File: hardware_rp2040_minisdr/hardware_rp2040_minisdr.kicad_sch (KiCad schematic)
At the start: 48 parts, among them IC1 PSA4-5043+, IC2 ADE-11X+, IC3 SI5351A-B-GTR, IC4 GALI-84+, IC5 ADCS7476AIMFX_NOPB, J1 Conn_Coaxial_Small, J2 USB_A, SW1 SW_Push, U1 RP2040, U2 W25Q128JVS, U3 AMS1117-3.3, Y1 Crystal_GND24, Y2 Crystal_GND24

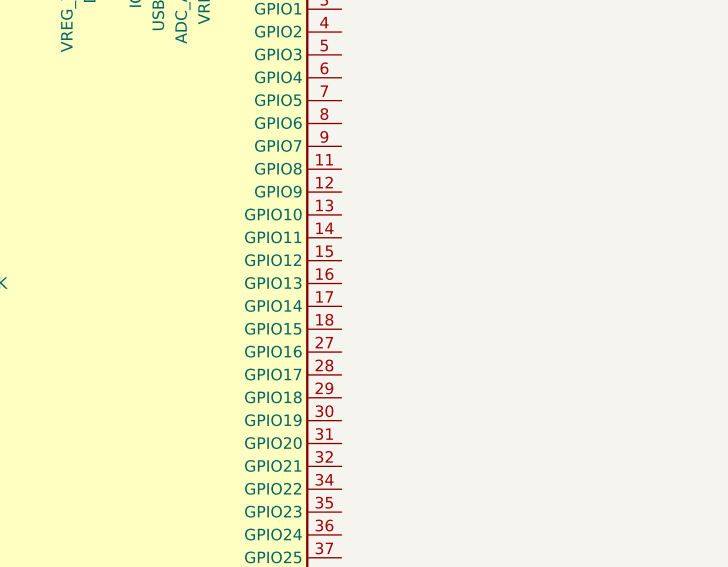
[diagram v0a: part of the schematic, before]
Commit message: board
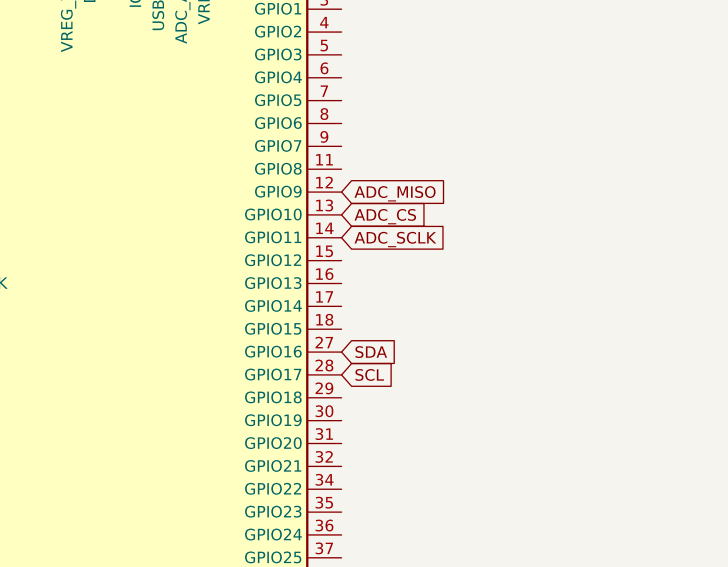
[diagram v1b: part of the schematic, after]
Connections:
- net ADC_CS: now also U1.13 (GPIO10)
- net ADC_MISO: now also U1.12 (GPIO9)
- net ADC_SCLK: now also U1.14 (GPIO11)
- net SCL: now also U1.28 (GPIO17)
- net SDA: now also U1.27 (GPIO16)
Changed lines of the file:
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@@
+		)
+	)
+	(global_label "ADC_SCLK"
+		(shape input)
+		(at 228.6 96.52 0)
+		(fields_autoplaced yes)
+		(effects
+			(font
+				(size 1.27 1.27)
+			)
+			(justify left)
+		)
+		(property "Intersheetrefs" "${INTERSHEET_REFS}"
+			(at 240.959 96.52 0)
+			(effects
+				(font
+					(size 1.27 1.27)
+				)
+				(justify left)
+				(hide yes)
+			)
 		)
 	)
@@
 		)
 	)
+	(global_label "ADC_CS"
+		(shape input)
+		(at 228.6 93.98 0)
+		(fields_autoplaced yes)
+		(effects
+			(font
+				(size 1.27 1.27)
+			)
+			(justify left)
+		)
+		(property "Intersheetrefs" "${INTERSHEET_REFS}"
+			(at 238.6609 93.98 0)
+			(effects
+				(font
+					(size 1.27 1.27)
+				)
+				(justify left)
+				(hide yes)
+			)
+		)
+	)
+	(global_label "SCL"
+		(shape input)
+		(at 228.6 111.76 0)
+		(fields_autoplaced yes)
+		(effects
+			(font
+				(size 1.27 1.27)
+			)
+			(justify left)
+		)
+		(property "Intersheetrefs" "${INTERSHEET_REFS}"
+			(at 235.0928 111.76 0)
+			(effects
+				(font
+					(size 1.27 1.27)
+				)
+				(justify left)
+				(hide yes)
+			)
+		)
+	)
+	(global_label "ADC_MISO"
+		(shape input)
+		(at 228.6 91.44 0)
+		(fields_autoplaced yes)
+		(effects
+			(font
+				(size 1.27 1.27)
+			)
+			(justify left)
+		)
+		(property "Intersheetrefs" "${INTERSHEET_REFS}"
+			(at 240.7776 91.44 0)
+			(effects
+				(font
+					(size 1.27 1.27)
+				)
+				(justify left)
+				(hide yes)
+			)
+		)
+	)
 	(global_label "GND"
 		(shape input)
@@
 				(hide yes)
 			)
+		)
+	)
+	(global_label "SDA"
+		(shape input)
+		(at 228.6 109.22 0)
+		(fields_autoplaced yes)
+		(effects
+			(font
+				(size 1.27 1.27)
+			)
+			(justify left)
+		)
+		(property "Intersheetrefs" "${INTERSHEET_REFS}"
+			(at 235.1533 109.22 0)
+			(effects
+				(font
+					(size 1.27 1.27)
+				)
+				(justify left)
+				(hide yes)
+			)

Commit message: board
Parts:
- C10, C11, C12, C13, C14, C15, C17, C18, C2, C20, C21, C23, C24, C25, C26, C3, C6, C7, C9: footprint (none) -> Capacitor_SMD:C_0402_1005Metric
- D1: footprint SOT95P280X145-5N -> (none)
- IC1: footprint PSA45043 -> (none)
- IC2: footprint SOTFL254P691X284-6N -> (none)
- IC3: footprint SOP50P490X110-10N -> (none)
- IC4: footprint GALI5 -> (none)
- IC5: footprint SOT95P280X145-6N -> (none)
- J1: footprint (none) -> Connector_Coaxial:SMA_Amphenol_132289_EdgeMount
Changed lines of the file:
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@@
 			)
 		)
-		(property "Footprint" "SOP50P490X110-10N"
+		(property "Footprint" ""
 			(at 153.67 243.51 0)
 			(effects
@@
 			)
 		)
-		(property "Footprint" ""
+		(property "Footprint" "Connector_Coaxial:SMA_Amphenol_132289_EdgeMount"
 			(at 29.21 106.68 0)
 			(effects
@@
 			)
 		)
-		(property "Footprint" ""
+		(property "Footprint" "Capacitor_SMD:C_0402_1005Metric"
 			(at 247.3452 44.45 0)
 			(effects
@@
 			)
 		)
-		(property "Footprint" ""
+		(property "Footprint" "Capacitor_SMD:C_0402_1005Metric"
 			(at 77.1652 130.81 0)
 			(effects
@@
 			)
 		)
-		(property "Footprint" ""
+		(property "Footprint" "Capacitor_SMD:C_0402_1005Metric"
 			(at 224.4852 44.45 0)
 			(effects
@@
 			)
 		)
-		(property "Footprint" "PSA45043"
+		(property "Footprint" ""
 			(at 45.72 14.3 0)
 			(effects
@@
 			)
 		)
-		(property "Footprint" "SOT95P280X145-5N"
+		(property "Footprint" ""
 			(at 55.88 172.39 0)
 			(effects
@@
 			)
 		)
-		(property "Footprint" ""
+		(property "Footprint" "Capacitor_SMD:C_0402_1005Metric"
 			(at 155.9052 133.35 0)
 			(effects
@@
 			)
 		)
-		(property "Footprint" "SOTFL254P691X284-6N"
+		(property "Footprint" ""
 			(at 72.39 213.03 0)
 			(effects
@@
 			)
 		)
-		(property "Footprint" ""
+		(property "Footprint" "Capacitor_SMD:C_0402_1005Metric"
 			(at 39.37 133.6548 0)
 			(effects
@@
 			)
 		)
-		(property "Footprint" ""
+		(property "Footprint" "Capacitor_SMD:C_0402_1005Metric"
 			(at 254.9652 44.45 0)
 			(effects
@@
 			)
 		)
-		(property "Footprint" "SOT95P280X145-6N"
+		(property "Footprint" ""
 			(at 66.04 251.13 0)
 			(effects
@@
 			)
 		)
-		(property "Footprint" ""
+		(property "Footprint" "Capacitor_SMD:C_0402_1005Metric"
 			(at 239.7252 44.45 0)
 			(effects
@@
 			)
 		)
-		(property "Footprint" "GALI5"
+		(property "Footprint" ""
 			(at 91.44 32.08 0)
 			(effects
@@
 			)
 		)
-		(property "Footprint" ""
+		(property "Footprint" "Capacitor_SMD:C_0402_1005Metric"
 			(at 262.5852 44.45 0)
 			(effects
@@
 			)
 		)
-		(property "Footprint" ""
+		(property "Footprint" "Capacitor_SMD:C_0402_1005Metric"
 			(at 187.6552 48.26 0)
 			(effects
@@
 			)
 		)
-		(property "Footprint" ""
+		(property "Footprint" "Capacitor_SMD:C_0402_1005Metric"
 			(at 29.5148 147.32 0)
 			(effects
@@
 			)
 		)
-		(property "Footprint" ""
+		(property "Footprint" "Capacitor_SMD:C_0402_1005Metric"
 			(at 108.9152 162.56 0)
 			(effects
@@
 			)
 		)
-		(property "Footprint" ""
+		(property "Footprint" "Capacitor_SMD:C_0402_1005Metric"
 			(at 195.2752 48.26 0)
 			(effects
@@
 			)
 		)
-		(property "Footprint" ""
+		(property "Footprint" "Capacitor_SMD:C_0402_1005Metric"
 			(at 216.8652 44.45 0)
 			(effects
@@
 			)
 		)
-		(property "Footprint" ""
+		(property "Footprint" "Capacitor_SMD:C_0402_1005Metric"
 			(at 38.1 105.7148 0)
 			(effects
@@
 			)
 		)
-		(property "Footprint" ""
+		(property "Footprint" "Capacitor_SMD:C_0402_1005Metric"
 			(at 106.68 108.2548 0)
 			(effects
@@
 			)
 		)
-		(property "Footprint" ""
+		(property "Footprint" "Capacitor_SMD:C_0402_1005Metric"
 			(at 132.3848 127 0)
 			(effects
@@
 			)
 		)
-		(property "Footprint" ""
+		(property "Footprint" "Capacitor_SMD:C_0402_1005Metric"
 			(at 108.9152 147.32 0)
 			(effects
@@
 			)
 		)
-		(property "Footprint" ""
+		(property "Footprint" "Capacitor_SMD:C_0402_1005Metric"
 			(at 232.1052 44.45 0)
 			(effects
@@
 			)
 		)
-		(property "Footprint" ""
+		(property "Footprint" "Capacitor_SMD:C_0402_1005Metric"
 			(at 155.9052 114.3 0)
 			(effects

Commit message: board
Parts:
- C16, C8: footprint (none) -> Capacitor_SMD:C_0402_1005Metric
- C19, C22, C4, C5: footprint (none) -> Capacitor_SMD:C_0805_2012Metric
- D1: footprint (none) -> user_imported_devices:ESDS314BVR_SOT95P280X145-5N
- IC1: footprint (none) -> user_imported_devices:PSA45043
- IC2: footprint (none) -> user_imported_devices:ADE-11X+_SOTFL254P691X284-6N
- IC3: footprint (none) -> user_imported_devices:SI5351_SOP50P490X110-10N
- IC4: footprint (none) -> user_imported_devices:GALI5
- IC5: footprint (none) -> user_imported_devices:ADCS7476_SOT95P280X145-6N
- L1, L2, L3, L4: footprint (none) -> Inductor_SMD:L_0805_2012Metric
- R2, R3, R4, R5, R6: footprint (none) -> Resistor_SMD:R_0402_1005Metric
- SW1: footprint (none) -> Button_Switch_SMD:SW_SPST_PTS810
- Y1, Y2: footprint (none) -> Crystal:Crystal_SMD_3225-4Pin_3.2x2.5mm
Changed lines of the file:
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@@
 			)
 		)
-		(property "Footprint" ""
+		(property "Footprint" "user_imported_devices:SI5351_SOP50P490X110-10N"
 			(at 153.67 243.51 0)
 			(effects
@@
 			)
 		)
-		(property "Footprint" ""
+		(property "Footprint" "Resistor_SMD:R_0402_1005Metric"
 			(at 171.45 126.238 90)
 			(effects
@@
 			)
 		)
-		(property "Footprint" ""
+		(property "Footprint" "user_imported_devices:PSA45043"
 			(at 45.72 14.3 0)
 			(effects
@@
 			)
 		)
-		(property "Footprint" ""
+		(property "Footprint" "user_imported_devices:ESDS314BVR_SOT95P280X145-5N"
 			(at 55.88 172.39 0)
 			(effects
@@
 			)
 		)
-		(property "Footprint" ""
+		(property "Footprint" "Capacitor_SMD:C_0402_1005Metric"
 			(at 192.7352 57.15 0)
 			(effects
@@
 			)
 		)
-		(property "Footprint" ""
+		(property "Footprint" "user_imported_devices:ADE-11X+_SOTFL254P691X284-6N"
 			(at 72.39 213.03 0)
 			(effects
@@
 			)
 		)
-		(property "Footprint" ""
+		(property "Footprint" "Resistor_SMD:R_0402_1005Metric"
 			(at 123.952 81.28 90)
 			(effects
@@
 			)
 		)
-		(property "Footprint" ""
+		(property "Footprint" "Capacitor_SMD:C_0805_2012Metric"
 			(at 84.1248 96.52 0)
 			(effects
@@
 			)
 		)
-		(property "Footprint" ""
+		(property "Footprint" "Inductor_SMD:L_0805_2012Metric"
 			(at 83.82 130.81 0)
 			(effects
@@
 			)
 		)
-		(property "Footprint" ""
+		(property "Footprint" "Capacitor_SMD:C_0805_2012Metric"
 			(at 67.0052 53.34 0)
 			(effects
@@
 			)
 		)
-		(property "Footprint" ""
+		(property "Footprint" "Capacitor_SMD:C_0402_1005Metric"
 			(at 218.1352 57.15 0)
 			(effects
@@
 			)
 		)
-		(property "Footprint" ""
+		(property "Footprint" "user_imported_devices:ADCS7476_SOT95P280X145-6N"
 			(at 66.04 251.13 0)
 			(effects
@@
 			)
 		)
-		(property "Footprint" ""
+		(property "Footprint" "Resistor_SMD:R_0402_1005Metric"
 			(at 168.91 80.518 90)
 			(effects
@@
 			)
 		)
-		(property "Footprint" ""
+		(property "Footprint" "Button_Switch_SMD:SW_SPST_PTS810"
 			(at 120.65 72.39 0)
 			(effects
@@
 			)
 		)
-		(property "Footprint" ""
+		(property "Footprint" "user_imported_devices:GALI5"
 			(at 91.44 32.08 0)
 			(effects
@@
 			)
 		)
-		(property "Footprint" ""
+		(property "Footprint" "Resistor_SMD:R_0402_1005Metric"
 			(at 85.852 135.89 90)
 			(effects
@@
 			)
 		)
-		(property "Footprint" ""
+		(property "Footprint" "Crystal:Crystal_SMD_3225-4Pin_3.2x2.5mm"
 			(at 107.95 151.13 0)
 			(effects
@@
 			)
 		)
-		(property "Footprint" ""
+		(property "Footprint" "Capacitor_SMD:C_0805_2012Metric"
 			(at 92.4052 53.34 0)
 			(effects
@@
 			)
 		)
-		(property "Footprint" ""
+		(property "Footprint" "Crystal:Crystal_SMD_3225-4Pin_3.2x2.5mm"
 			(at 154.94 120.65 0)
 			(effects
@@
 			)
 		)
-		(property "Footprint" ""
+		(property "Footprint" "Capacitor_SMD:C_0805_2012Metric"
 			(at 80.01 140.6652 0)
 			(effects
@@
 			)
 		)
-		(property "Footprint" ""
+		(property "Footprint" "Inductor_SMD:L_0805_2012Metric"
 			(at 30.48 129.54 0)
 			(effects
@@
 			)
 		)
-		(property "Footprint" ""
+		(property "Footprint" "Inductor_SMD:L_0805_2012Metric"
 			(at 93.98 100.33 0)
 			(effects
@@
 			)
 		)
-		(property "Footprint" ""
+		(property "Footprint" "Inductor_SMD:L_0805_2012Metric"
 			(at 30.48 139.7 0)
 			(effects
@@
 			)
 		)
-		(property "Footprint" ""
+		(property "Footprint" "Resistor_SMD:R_0402_1005Metric"
 			(at 168.91 74.422 90)
 			(effects
